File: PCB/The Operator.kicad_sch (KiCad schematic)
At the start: 23 parts, among them SW1 SW_Push, SW2 SW_Push, SW3 SW_Push, SW4 SW_Push, SW5 RotaryEncoder_Switch, U1 MOUDLE-SEEEDUINO-XIAO

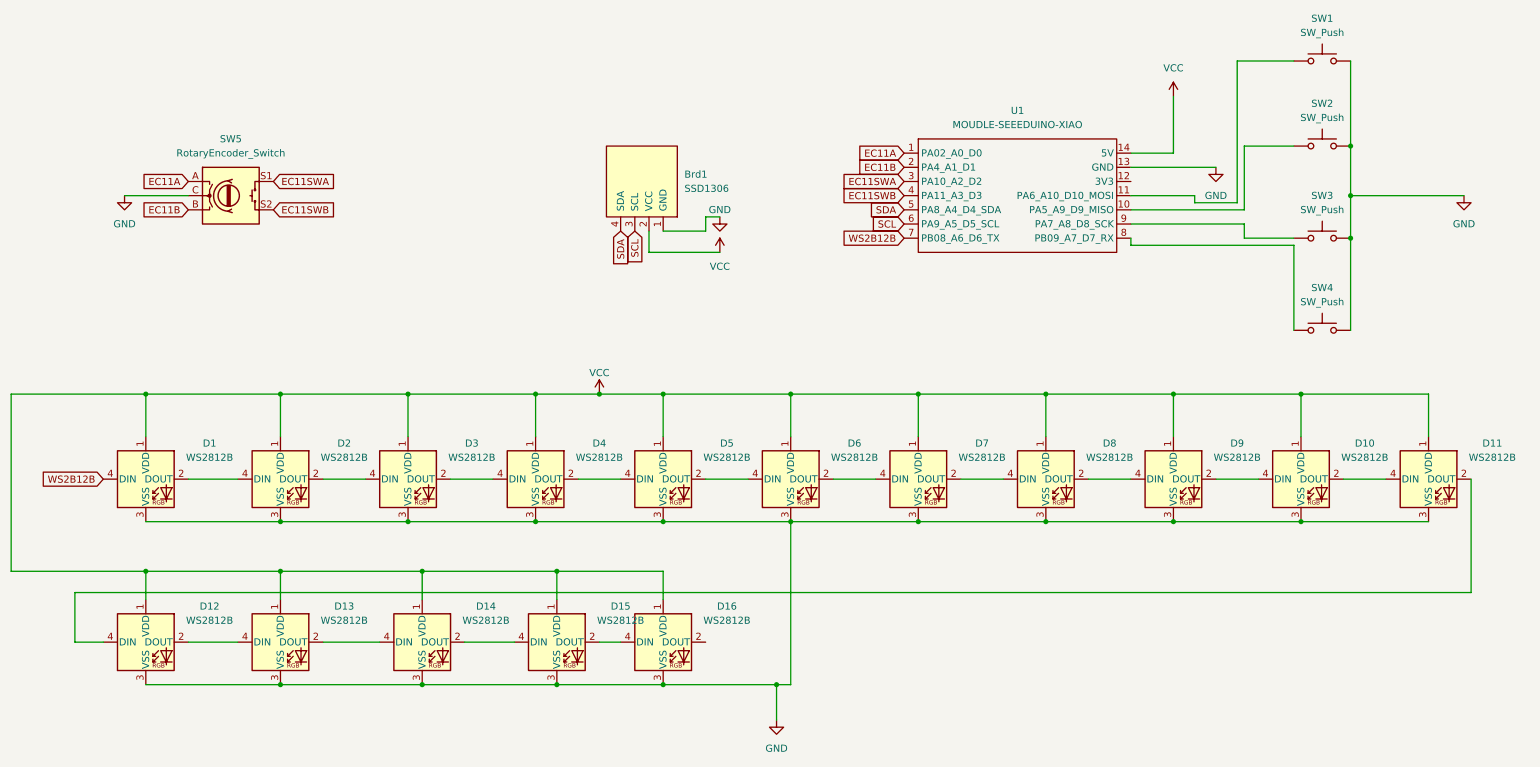
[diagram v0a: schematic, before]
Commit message: fixed leds
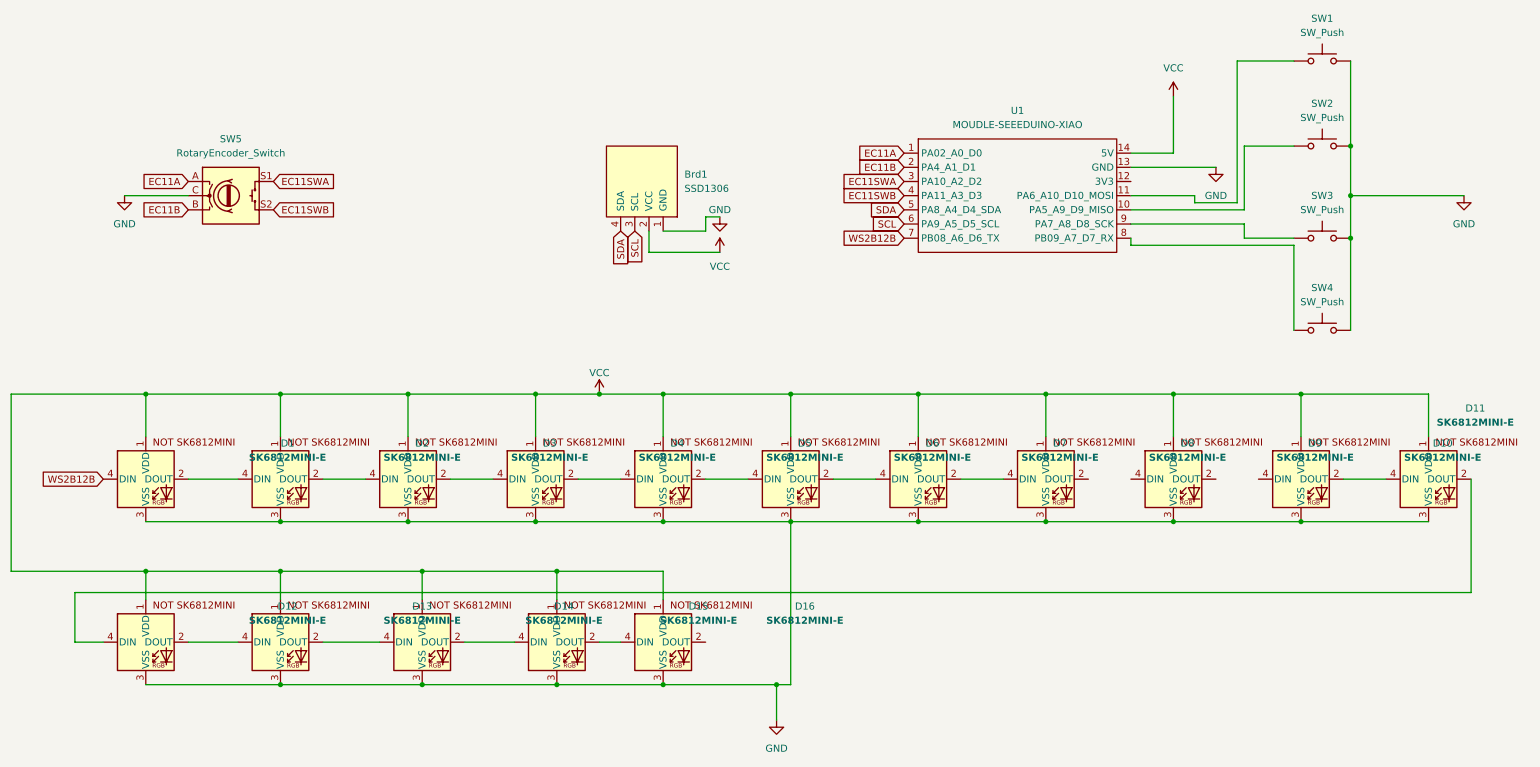
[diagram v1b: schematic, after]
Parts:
- removed D1, D10, D11, D12, D13, D14, D15, D16, D2, D3, D4, D5, D6, D7, D8, D9: WS2812B, LED_SMD:LED_WS2812B_PLCC4_5.0x5.0mm_P3.2mm, symbol LED:WS2812B
- added D1, D10, D11, D12, D13, D14, D15, D16, D2, D3, D4, D5, D6, D7, D8, D9: SK6812MINI-E, SK6812MINI-E - 3.2x2.8x1.78mm, symbol SK6812MINI-E:SK6812MINI-E
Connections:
- net GND: now also D1.3 (VSS), D10.3 (VSS), D11.3 (VSS), D12.3 (VSS), D13.3 (VSS), D14.3 (VSS), D15.3 (VSS), D16.3 (VSS), D2.3 (VSS), D3.3 (VSS), D4.3 (VSS), D5.3 (VSS), D6.3 (VSS), D7.3 (VSS), D8.3 (VSS), D9.3 (VSS)
- net VCC: now also D1.1 (VDD), D10.1 (VDD), D11.1 (VDD), D12.1 (VDD), D13.1 (VDD), D14.1 (VDD), D15.1 (VDD), D16.1 (VDD), D2.1 (VDD), D3.1 (VDD), D4.1 (VDD), D5.1 (VDD), D6.1 (VDD), D7.1 (VDD), D8.1 (VDD), D9.1 (VDD)
- net WS2B12B: now also D1.4 (DIN)
- new net: D10.2 (DOUT), D11.4 (DIN)
- new net: D13.2 (DOUT), D14.4 (DIN)
- new net: D12.2 (DOUT), D13.4 (DIN)
- new net: D1.2 (DOUT), D2.4 (DIN)
- new net: D3.2 (DOUT), D4.4 (DIN)
- new net: D2.2 (DOUT), D3.4 (DIN)
- new net: D7.2 (DOUT), D8.4 (DIN)
- new net: D6.2 (DOUT), D7.4 (DIN)
- new net: D4.2 (DOUT), D5.4 (DIN)
- new net: D11.2 (DOUT), D12.4 (DIN)
- new net: D15.2 (DOUT), D16.4 (DIN)
- new net: D14.2 (DOUT), D15.4 (DIN)
- new net: D5.2 (DOUT), D6.4 (DIN)
